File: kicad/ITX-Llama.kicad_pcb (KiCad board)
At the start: 4 copper layers, 188 x 188 mm, 421 parts, among them J1 ATX_POWER, J10 SATA, J11 SPEAKER, J12 MSD, J14 AUDIO, J15 KBC, J16 KBD, J17 USB_ETH, J18 USB_HID, J19 HID_POWER, J2 MICRO_SD, J20 FAN1, J21 FAN2, J22 GAMEPORT, J23 WAVETABLE, J24 PI_ZERO2, J25 POWER, J26 LEFT, J27 RIGHT, J28 COM2_TTL, J29 PI_2/3/4, J3 FRONT_PANEL, J30 FAN3, J31 FAN1_VDD, J32 FAN2_VDD, J33 FAN3_VDD, J34 CD_IN, J35 D1_MINI, J36 ESP_POWER, J38 J_TOSLINK_ZGY133T10, J39 LINE_L, J4 PS/2, J40 LINE_R, J41 EXT_SYNTH, J42 PI_I2C, J43 I2C, J46 RP_DEBUG, J5 AGP_3.3V, J6 CLICK_VOL, J7 MSC, J8 COM1, J9 INT_SPKR_VOL, P1 P_SOM-128-EX, Q1 NPN, Q10 Q_NMOS_GDS, Q11 Q_NMOS_GDS, Q2 NPN, Q3 NPN, Q4 NPN, Q5 NPN, Q6 NPN, Q7 NPN, Q8 Q_NMOS_GDS, Q9 Q_NMOS_GDS, SW1 POWER, SW2 RESET, SW3 CH559_PRG, T1 Pulse_H1102NL, U1 MAX16054, U10 U_MIC5219-3.3YM5, U11 EMC2303, U12 PCM5102A, U13 U_MIC5219-3.3YM5, U14 U_MIC5219-3.3YM5, U15 W25Q32JVSS, U16 U_74LVC1G126, U17 U_RP2040, U2 U_74LVC1G04, U3 U_CS4237B-KQ, U4 GD75232, U5 U_MC33078, U6 PI7C9X118SL, U7 AP7165, U8 U_MIC5219-3.3YM5, U9 U_ATTINY84A, X1 16.9344MHz, X2 12MHz

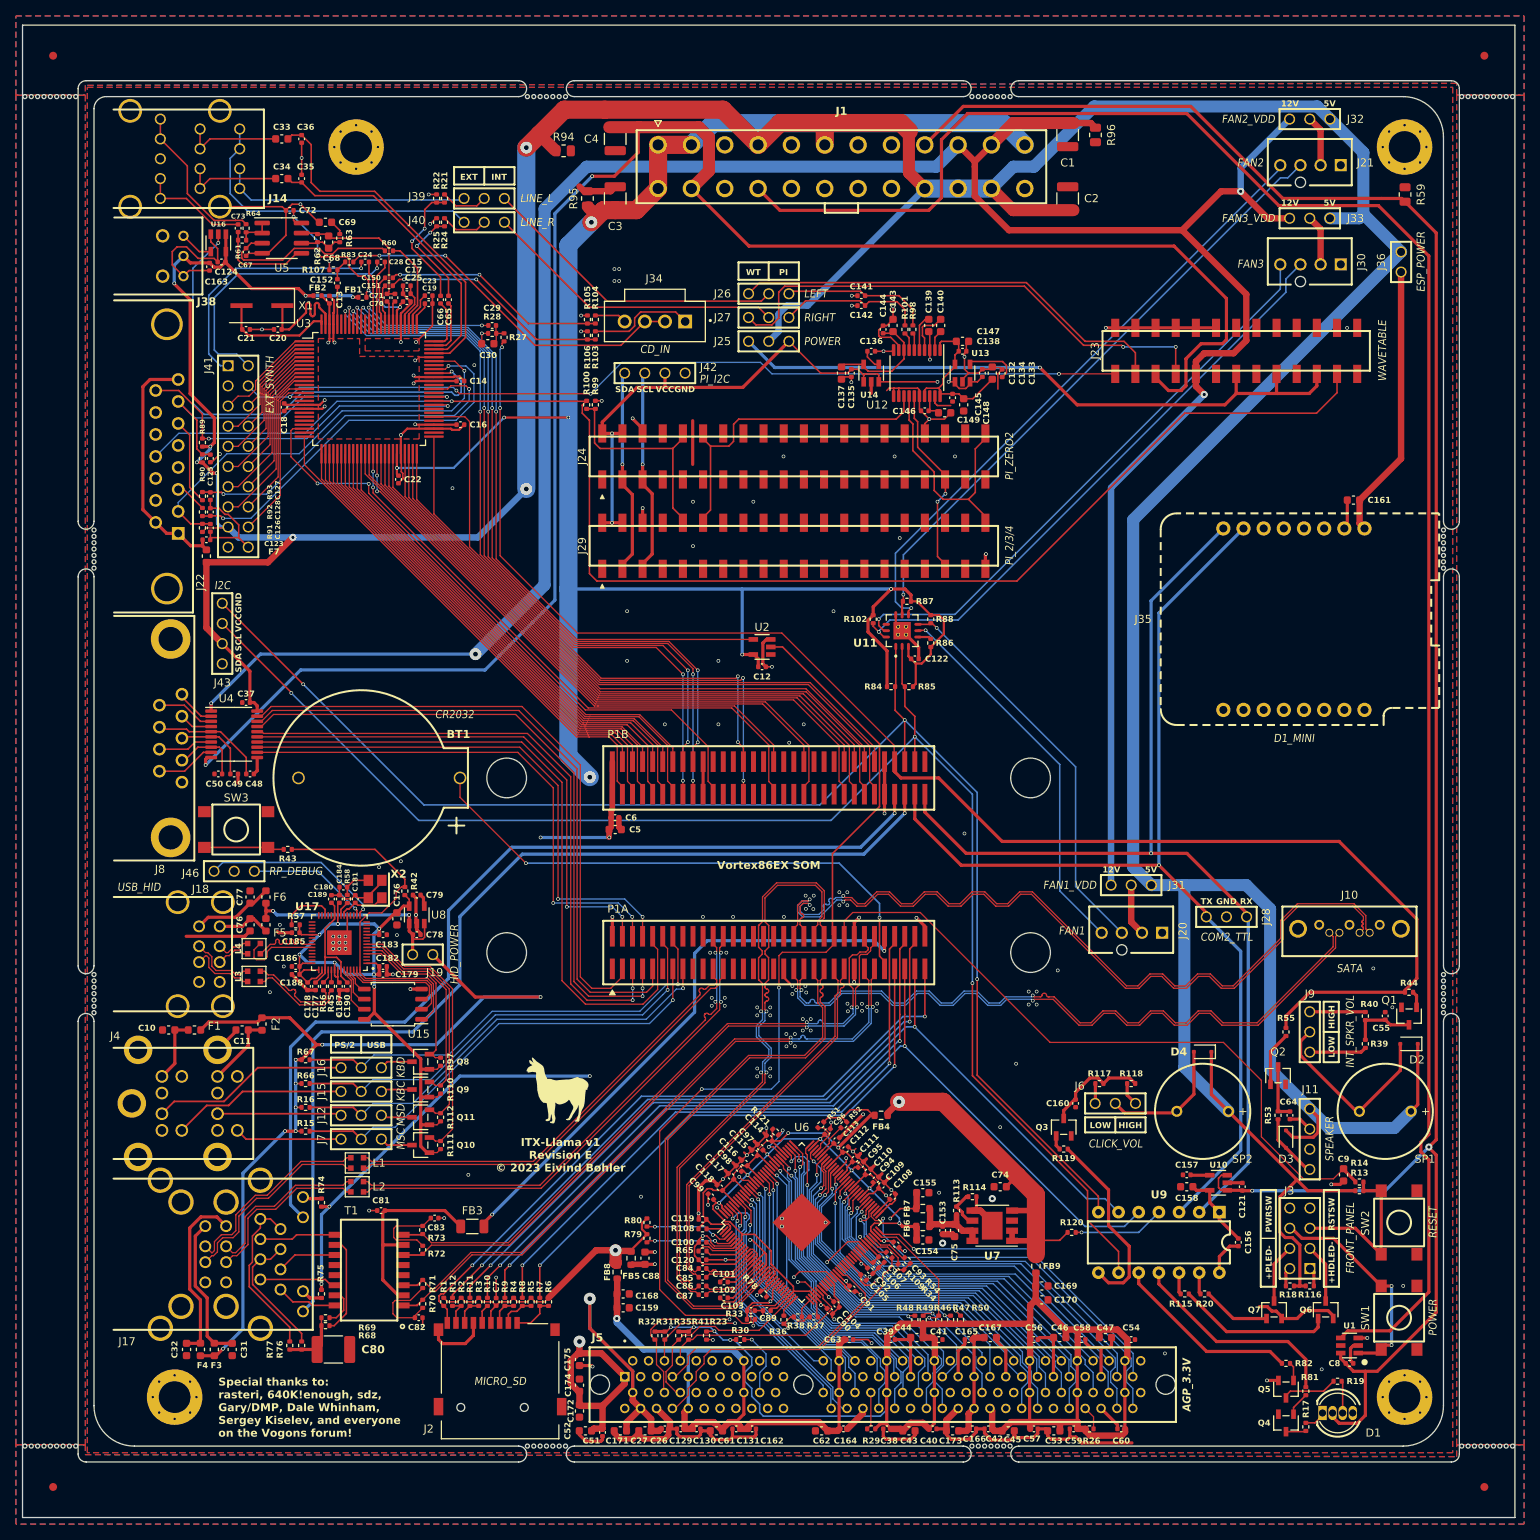
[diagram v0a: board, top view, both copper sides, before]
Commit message: revK
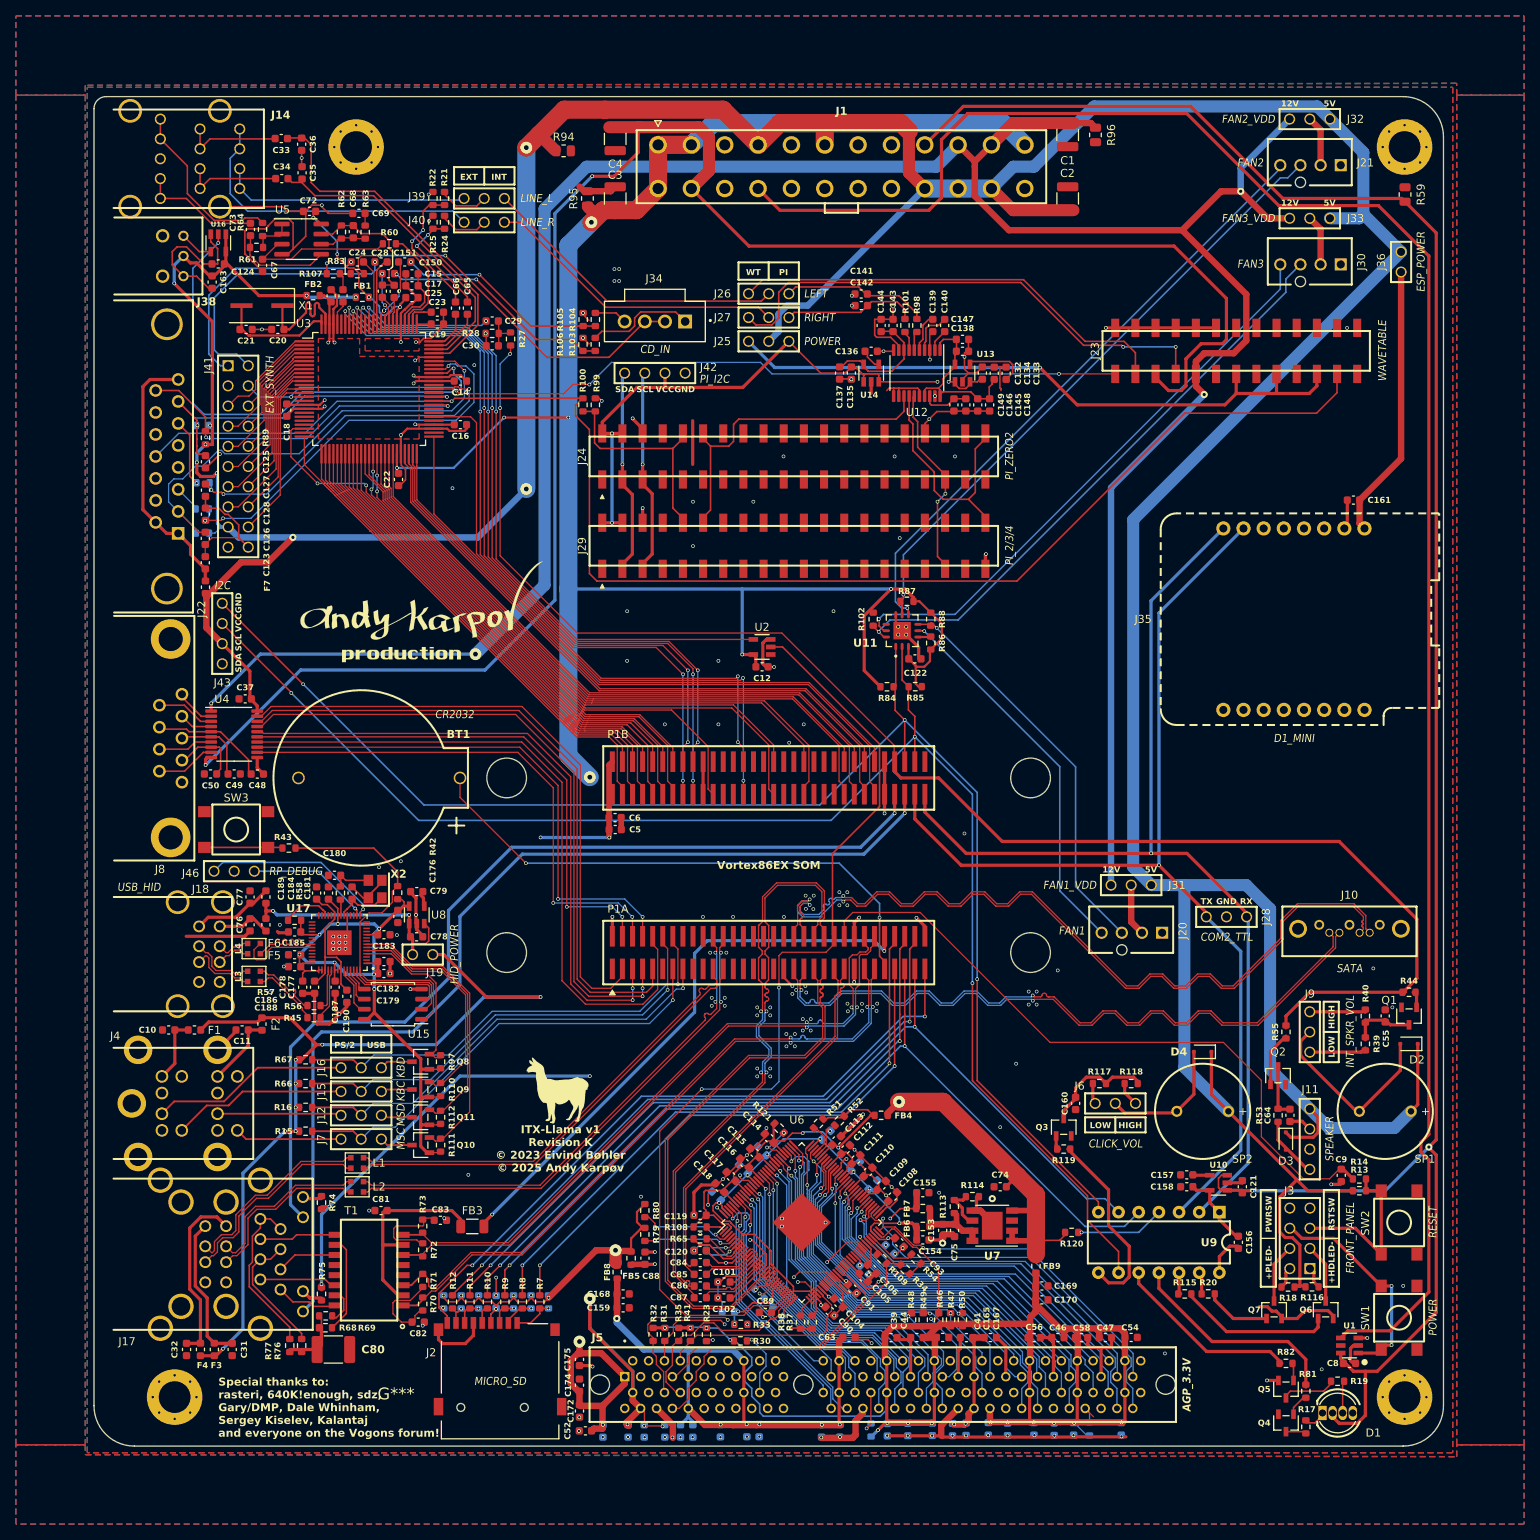
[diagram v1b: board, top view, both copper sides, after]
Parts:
- added G***: LOGO, footprints:andy_karpov_logo4_silk, F.Cu at (31.2, -99.0)
- added G***: LOGO, footprints:karabas_qr_12, B.Cu at (27.9, -0.41)
- C100, C103, C107, C129, C130, C131, C162, C164, C166, C26, C38, C40, C42, C51, C57, C59, C60, C7, C92, C94, C95, C96, C97, C98, C99: footprint llama_shared:C_0402_1005Metric -> llama_shared:C_0603_1608Metric; moved to B.Cu
- C101, C102, C104, C105, C106, C108, C109, C110, C111, C112, C113, C114, C115, C116, C117, C118, C119, C12, C120, C121, C122, C123, C124, C125, C126, C127, C128, C13, C132, C133, C135, C136, C138, C14, C141, C142, C144, C145, C146, C15, C150, C151, C152, C153, C156, C157, C16, C160, C163, C165, C17, C177, C178, C179, C18, C180, C181, C182, C183, C184, C185, C186, C187, C188, C189, C19, C190, C20, C21, C22, C23, C24, C25, C28, C29, C35, C36, C37, C39, C41, C48, C49, C50, C54, C55, C56, C58, C6, C63, C64, C65, C66, C67, C70, C71, C72, C73, C78, C79, C8, C81, C82, C83, C84, C85, C86, C87, C89, C90, C91, C93: footprint llama_shared:C_0402_1005Metric -> llama_shared:C_0603_1608Metric
- C171, C173, C27, C43, C45, C53, C61, C62: moved to B.Cu
- FB1, FB2, R10, R100, R101, R102, R103, R104, R105, R106, R107, R108, R109, R11, R110, R111, R112, R113, R114, R115, R116, R117, R118, R119, R12, R120, R121, R13, R14, R15, R16, R17, R18, R19, R20, R21, R22, R23, R24, R25, R27, R28, R30, R31, R32, R33, R34, R35, R37, R38, R39, R40, R41, R42, R43, R44, R45, R46, R47, R48, R49, R50, R51, R52, R53, R54, R55, R56, R57, R58, R60, R61, R62, R63, R64, R65, R66, R67, R68, R69, R7, R70, R71, R72, R73, R74, R75, R76, R77, R79, R8, R80, R81, R82, R83, R84, R85, R86, R87, R88, R89, R9, R97, R98, R99: footprint llama_shared:R_0402_1005Metric -> llama_shared:R_0603_1608Metric
- R1, R2, R26, R29, R3, R36, R4, R5, R6, R78, R90, R91, R92, R93: footprint llama_shared:R_0402_1005Metric -> llama_shared:R_0603_1608Metric; moved to B.Cu
- moved C146 5.22 mm to (99.7, -125.0), turned to 90 degrees
- moved R45 4.52 mm to (17.6, -47.8), turned to 0 degrees
- moved C69 4.36 mm to (23.2, -149.1)
- moved R90 4.15 mm to (3.53, -122.4), turned to 180 degrees
- moved F7 3.92 mm to (3.89, -102.0)
- moved C68 3.37 mm to (22.5, -146.8)
- moved C145 3.30 mm to (101.2, -125.0)
- moved R63 3.29 mm to (24.0, -146.8)
- moved C148 3.27 mm to (102.7, -125.0)
- moved R62 3.10 mm to (21.0, -146.8)
- moved C123 2.90 mm to (3.86, -105.1), turned to -90 degrees
- moved C103 2.85 mm to (69.7, -10.8), turned to 0 degrees
- moved C150 2.82 mm to (29.0, -143.0)
- moved C19 2.80 mm to (33.1, -135.2)
- moved R56 2.70 mm to (17.6, -49.3), turned to 0 degrees
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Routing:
- net unconnected-(J17-Shield-PadS)_5: track 43.0 -> 0.00 mm
- net unconnected-(J17-Shield-PadS): track 0.00 -> 43.0 mm
- net GND: track 560.0 -> 536.8 mm, vias 170 -> 202
- net +3.3V_118SL: track 154.0 -> 162.0 mm, vias 9 -> 12
- net /JAB1: track 55.1 -> 62.0 mm
- net Net-(U17-USB_DP): track 1.55 -> 6.58 mm
- net +3.3V: track 484.4 -> 489.1 mm, vias 12 -> 19
- net Net-(U5A-+): track 23.2 -> 19.2 mm
- net /USBHID1-: track 11.8 -> 8.30 mm
- net Net-(U17-USB_DM): track 1.80 -> 5.32 mm
- net RP_3.3V: track 98.6 -> 95.1 mm
- net +1.15V_VDDC: track 106.0 -> 102.5 mm, vias 11 -> 12
- net /USBHID1+: track 11.9 -> 8.54 mm
- net /USB_KBCLK_LV: track 26.0 -> 29.1 mm
- net VCC: track 902.1 -> 899.0 mm, vias 20 -> 24
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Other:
- board size 188 x 188 mm -> 170 x 170 mm
- board text added: "ITX-Llama v1 Revision K © 2023 Eivind Bøhler © 2025 Andy Karpøv"
- board text added: "Special thanks to: rasteri, 640K!enough, sdz, Gary/DMP, Dale Whinham, Sergey Kiselev, Kalantaj and everyone on the Vogons forum!"
- board text removed: "ITX-Llama v1 Revision E © 2023 Eivind Bøhler"
- board text removed: "Special thanks to: rasteri, 640K!enough, sdz, Gary/DMP, Dale Whinham, Sergey Kiselev, and everyone on the Vogons forum!"
